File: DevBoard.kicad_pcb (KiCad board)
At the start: 2 copper layers, 26.6 x 51 mm, 38 parts, among them J1 USB_C_Receptacle_USB2.0_14P, J2 Conn_01x20_Pin, J3 Conn_01x20_Pin, J5 Conn_01x20_Pin, J6 Conn_01x03_Pin, J7 Conn_01x20_Pin, SW1 SW_Push, U1 RP2040, U2 NCP1117-3.3_SOT223, U3 W25Q128JVS, Y1 12 MHz

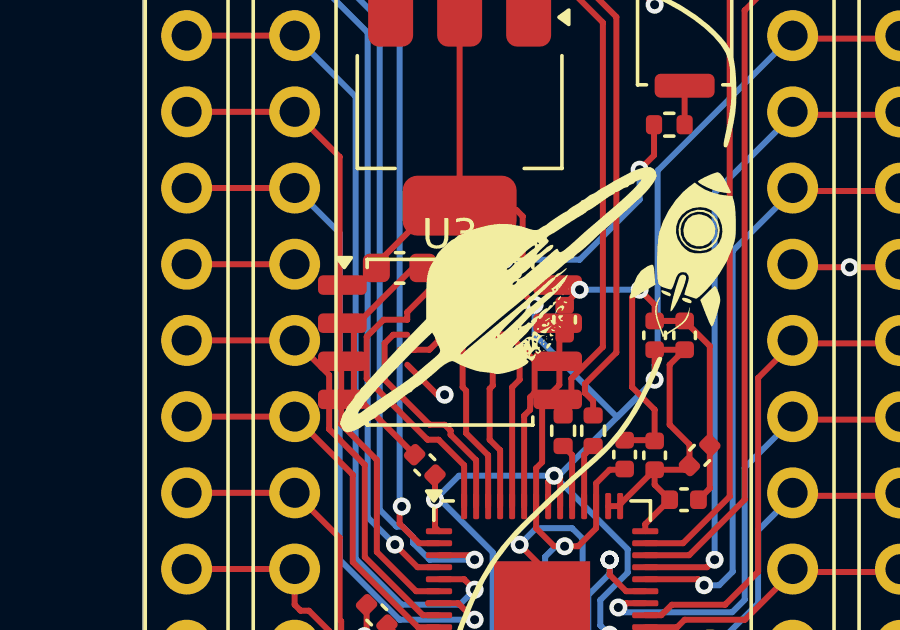
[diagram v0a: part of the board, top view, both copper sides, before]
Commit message: Add files via upload
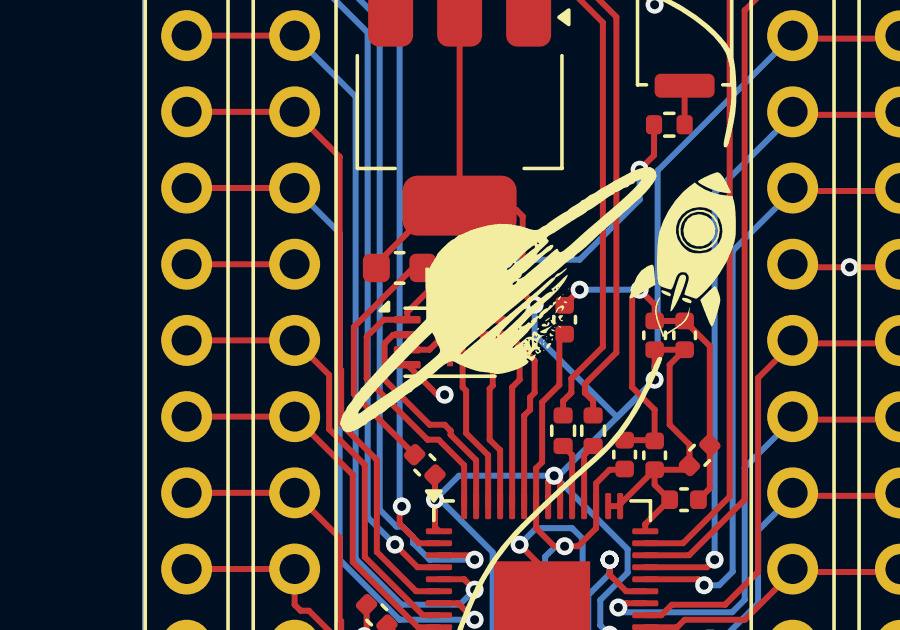
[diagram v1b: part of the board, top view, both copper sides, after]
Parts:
- U3: footprint Package_SO:SOIC-8_5.3x5.3mm_P1.27mm -> Package_SON:Winbond_USON-8-1EP_3x2mm_P0.5mm_EP0.2x1.6mm
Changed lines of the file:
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@@
 		)
 	)
-	(footprint "Package_SO:SOIC-8_5.3x5.3mm_P1.27mm"
+	(footprint "Package_SON:Winbond_USON-8-1EP_3x2mm_P0.5mm_EP0.2x1.6mm"
 		(layer "F.Cu")
 		(at 97.679 132.75)
-		(descr "SOIC, 8 Pin (JEITA/EIAJ ED-7311-19 variation 08-001-BBA and Atmel/Microchip, 208 mils width, https://www.jeita.or.jp/japanese/standard/book/ED-7311-19/#target/page_no=21, https://ww1.microchip.com/downloads/en/DeviceDoc/20005045C.pdf#page=23, https://ww1.microchip.com/downloads/en/DeviceDoc/doc2535.pdf#page=162), generated with kicad-footprint-generator ipc_gullwing_generator.py")
-		(tags "SOIC SO P-SOP SOP SOP-8 SO SO-8 8S2 S2AE/F K04-056 CASE-751BE SO8W 8-Pin-SOIC PSA W8-2 W8-4 W8MS-1 FPT-8P-M08")
+		(descr "Winbond  USON, 8 Pin (https://www.lcsc.com/datasheet/lcsc_datasheet_2205122030_Winbond-Elec-W25Q16JVUXIQ_C2843335.pdf#page=66f), generated with kicad-footprint-generator ipc_noLead_generator.py")
+		(tags "Winbond USON NoLead")
 		(property "Reference" "U3"
-			(at 0 -3.6 0)
+			(at 0 -1.95 0)
 			(layer "F.SilkS")
 			(effects
@@
 		)
 		(property "Value" "W25Q128JVS"
-			(at 0 3.6 0)
+			(at 0 1.95 0)
 			(layer "F.Fab")
 			(effects
@@
 		(attr smd)
 		(fp_line
-			(start -2.76 -2.76)
-			(end -2.76 -2.49)
+			(start -1.5 -1.135)
+			(end 1.5 -1.135)
 			(stroke
 				(width 0.12)
@@
 		)
 		(fp_line
-			(start -2.76 2.76)
-			(end -2.76 2.49)
-			(stroke
-				(width 0.12)
-				(type solid)
-			)
-			(layer "F.SilkS")
-		)
-		(fp_line
-			(start 0 -2.76)
-			(end -2.76 -2.76)
-			(stroke
-				(width 0.12)
-				(type solid)
-			)
-			(layer "F.SilkS")
-		)
-		(fp_line
-			(start 0 -2.76)
-			(end 2.76 -2.76)
-			(stroke
-				(width 0.12)
-				(type solid)
-			)
-			(layer "F.SilkS")
-		)
-		(fp_line
-			(start 0 2.76)
-			(end -2.76 2.76)
-			(stroke
-				(width 0.12)
-				(type solid)
-			)
-			(layer "F.SilkS")
-		)
-		(fp_line
-			(start 0 2.76)
-			(end 2.76 2.76)
-			(stroke
-				(width 0.12)
-				(type solid)
-			)
-			(layer "F.SilkS")
-		)
-		(fp_line
-			(start 2.76 -2.76)
-			(end 2.76 -2.49)
-			(stroke
-				(width 0.12)
-				(type solid)
-			)
-			(layer "F.SilkS")
-		)
-		(fp_line
-			(start 2.76 2.76)
-			(end 2.76 2.49)
+			(start -1.5 1.135)
+			(end 1.5 1.135)
 			(stroke
 				(width 0.12)
@@
 		(fp_poly
 			(pts
-				(xy -3.525 -2.49) (xy -3.765 -2.82) (xy -3.285 -2.82)
+				(xy -2.05 -1.05) (xy -2.33 -1.05) (xy -2.05 -1.33)
 			)
 			(stroke
@@
 		)
 		(fp_line
-			(start -4.65 -2.48)
-			(end -2.9 -2.48)
-			(stroke
-				(width 0.05)
-				(type solid)
-			)
-			(layer "F.CrtYd")
-		)
-		(fp_line
-			(start -4.65 2.48)
-			(end -4.65 -2.48)
-			(stroke
-				(width 0.05)
-				(type solid)
-			)
-			(layer "F.CrtYd")
-		)
-		(fp_line
-			(start -2.9 -2.9)
-			(end 2.9 -2.9)
-			(stroke
-				(width 0.05)
-				(type solid)
-			)
-			(layer "F.CrtYd")
-		)
-		(fp_line
-			(start -2.9 -2.48)
-			(end -2.9 -2.9)
-			(stroke
-				(width 0.05)
-				(type solid)
-			)
-			(layer "F.CrtYd")
-		)
-		(fp_line
-			(start -2.9 2.48)
-			(end -4.65 2.48)
-			(stroke
-				(width 0.05)
-				(type solid)
-			)
-			(layer "F.CrtYd")
-		)
-		(fp_line
-			(start -2.9 2.9)
-			(end -2.9 2.48)
-			(stroke
-				(width 0.05)
-				(type solid)
-			)
-			(layer "F.CrtYd")
-		)
-		(fp_line
-			(start 2.9 -2.9)
-			(end 2.9 -2.48)
-			(stroke
-				(width 0.05)
-				(type solid)
-			)
-			(layer "F.CrtYd")
-		)
-		(fp_line
-			(start 2.9 -2.48)
-			(end 4.65 -2.48)
-			(stroke
-				(width 0.05)
-				(type solid)
-			)
-			(layer "F.CrtYd")
-		)
-		(fp_line
-			(start 2.9 2.48)
-			(end 2.9 2.9)
-			(stroke
-				(width 0.05)
-				(type solid)
-			)
-			(layer "F.CrtYd")
-		)
-		(fp_line
-			(start 2.9 2.9)
-			(end -2.9 2.9)
-			(stroke
-				(width 0.05)
-				(type solid)
-			)
-			(layer "F.CrtYd")
-		)
-		(fp_line
-			(start 4.65 -2.48)
-			(end 4.65 2.48)
-			(stroke
-				(width 0.05)
-				(type solid)
-			)
-			(layer "F.CrtYd")
-		)
-		(fp_line
-			(start 4.65 2.48)
-			(end 2.9 2.48)
-			(stroke
-				(width 0.05)
-				(type solid)
-			)
-			(layer "F.CrtYd")
-		)
-		(fp_line
-			(start -2.65 -1.65)
-			(end -1.65 -2.65)
+			(start -2.13 -1.13)
+			(end -1.75 -1.13)
+			(stroke
+				(width 0.05)
+				(type solid)
+			)
+			(layer "F.CrtYd")
+		)
+		(fp_line
+			(start -2.13 1.13)
+			(end -2.13 -1.13)
+			(stroke
+				(width 0.05)
+				(type solid)
+			)
+			(layer "F.CrtYd")
+		)
+		(fp_line
+			(start -1.75 -1.25)
+			(end 1.75 -1.25)
+			(stroke
+				(width 0.05)
+				(type solid)
+			)
+			(layer "F.CrtYd")
+		)
+		(fp_line
+			(start -1.75 -1.13)
+			(end -1.75 -1.25)
+			(stroke
+				(width 0.05)
+				(type solid)
+			)
+			(layer "F.CrtYd")
+		)
+		(fp_line
+			(start -1.75 1.13)
+			(end -2.13 1.13)
+			(stroke
+				(width 0.05)
+				(type solid)
+			)
+			(layer "F.CrtYd")
+		)
+		(fp_line
+			(start -1.75 1.25)
+			(end -1.75 1.13)
+			(stroke
+				(width 0.05)
+				(type solid)
+			)
+			(layer "F.CrtYd")
+		)
+		(fp_line
+			(start 1.75 -1.25)
+			(end 1.75 -1.13)
+			(stroke
+				(width 0.05)
+				(type solid)
+			)
+			(layer "F.CrtYd")
+		)
+		(fp_line
+			(start 1.75 -1.13)
+			(end 2.13 -1.13)
+			(stroke
+				(width 0.05)
+				(type solid)
+			)
+			(layer "F.CrtYd")
+		)
+		(fp_line
+			(start 1.75 1.13)
+			(end 1.75 1.25)
+			(stroke
+				(width 0.05)
+				(type solid)
+			)
+			(layer "F.CrtYd")
+		)
+		(fp_line
+			(start 1.75 1.25)
+			(end -1.75 1.25)
+			(stroke
+				(width 0.05)
+				(type solid)
+			)
+			(layer "F.CrtYd")
+		)
+		(fp_line
+			(start 2.13 -1.13)
+			(end 2.13 1.13)
+			(stroke
+				(width 0.05)
+				(type solid)
+			)
+			(layer "F.CrtYd")
+		)
+		(fp_line
+			(start 2.13 1.13)
+			(end 1.75 1.13)
+			(stroke
+				(width 0.05)
+				(type solid)
+			)
+			(layer "F.CrtYd")
+		)
+		(fp_poly
+			(pts
+				(xy -1.5 -0.5) (xy -1.5 1) (xy 1.5 1) (xy 1.5 -1) (xy -1 -1)
+			)
 			(stroke
 				(width 0.1)
 				(type solid)
 			)
-			(layer "F.Fab")
-		)
-		(fp_line
-			(start -2.65 2.65)
-			(end -2.65 -1.65)
-			(stroke
-				(width 0.1)
-				(type solid)
-			)
-			(layer "F.Fab")
-		)
-		(fp_line
-			(start -1.65 -2.65)
-			(end 2.65 -2.65)
-			(stroke
-				(width 0.1)
-				(type solid)
-			)
-			(layer "F.Fab")
-		)
-		(fp_line
-			(start 2.65 -2.65)
-			(end 2.65 2.65)
-			(stroke
-				(width 0.1)
-				(type solid)
-			)
-			(layer "F.Fab")
-		)
-		(fp_line
-			(start 2.65 2.65)
-			(end -2.65 2.65)
-			(stroke
-				(width 0.1)
-				(type solid)
-			)
+			(fill no)
 			(layer "F.Fab")
 		)
@@
 			(effects
 				(font
-					(size 1 1)
-					(thickness 0.15)
-				)
-			)
+					(size 0.75 0.75)
+					(thickness 0.11)
+				)
+			)
+		)
+		(pad "" smd roundrect
+			(at 0 0)
+			(size 0.16 1.29)
+			(layers "F.Paste")
+			(roundrect_rratio 0.25)
 		)
 		(pad "1" smd roundrect
-			(at -3.5875 -1.905)
-			(size 1.625 0.65)
+			(at -1.425 -0.75)
+			(size 0.9 0.25)
 			(layers "F.Cu" "F.Mask" "F.Paste")
 			(roundrect_rratio 0.25)
@@
 		)
 		(pad "2" smd roundrect
-			(at -3.5875 -0.635)
-			(size 1.625 0.65)
+			(at -1.425 -0.25)
+			(size 0.9 0.25)
 			(layers "F.Cu" "F.Mask" "F.Paste")
 			(roundrect_rratio 0.25)
@@
 		)
 		(pad "3" smd roundrect
-			(at -3.5875 0.635)
-			(size 1.625 0.65)
+			(at -1.425 0.25)
+			(size 0.9 0.25)
 			(layers "F.Cu" "F.Mask" "F.Paste")
 			(roundrect_rratio 0.25)
@@
 		)
 		(pad "4" smd roundrect
-			(at -3.5875 1.905)
-			(size 1.625 0.65)
+			(at -1.425 0.75)
+			(size 0.9 0.25)
 			(layers "F.Cu" "F.Mask" "F.Paste")
 			(roundrect_rratio 0.25)
@@
 		)
 		(pad "5" smd roundrect
-			(at 3.5875 1.905)
-			(size 1.625 0.65)
+			(at 1.425 0.75)
+			(size 0.9 0.25)
 			(layers "F.Cu" "F.Mask" "F.Paste")
 			(roundrect_rratio 0.25)
@@
 		)
 		(pad "6" smd roundrect
-			(at 3.5875 0.635)
-			(size 1.625 0.65)
+			(at 1.425 0.25)
+			(size 0.9 0.25)
 			(layers "F.Cu" "F.Mask" "F.Paste")
 			(roundrect_rratio 0.25)
@@
 		)
 		(pad "7" smd roundrect
-			(at 3.5875 -0.635)
-			(size 1.625 0.65)
+			(at 1.425 -0.25)
+			(size 0.9 0.25)
 			(layers "F.Cu" "F.Mask" "F.Paste")
 			(roundrect_rratio 0.25)
@@
 		)
 		(pad "8" smd roundrect
-			(at 3.5875 -1.905)
-			(size 1.625 0.65)
+			(at 1.425 -0.75)
+			(size 0.9 0.25)
 			(layers "F.Cu" "F.Mask" "F.Paste")
 			(roundrect_rratio 0.25)
@@
 			(pintype "power_in")
 		)
+		(pad "9" smd rect
+			(at 0 0)
+			(size 0.2 1.6)
+			(property pad_prop_heatsink)
+			(layers "F.Cu" "F.Mask")
+			(zone_connect 2)
+		)
 		(embedded_fonts no)
-		(model "${KICAD9_3DMODEL_DIR}/Package_SO.3dshapes/SOIC-8_5.3x5.3mm_P1.27mm.step"
+		(model "${KICAD9_3DMODEL_DIR}/Package_SON.3dshapes/Winbond_USON-8-1EP_3x2mm_P0.5mm_EP0.2x1.6mm.step"
 			(offset
 				(xyz 0 0 0)
